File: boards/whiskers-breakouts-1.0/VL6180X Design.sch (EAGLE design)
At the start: 12 parts, among them J1 FEMALE 2x3, Q3 BSS138, Q4 BSS138, U1 VL6180X, U2 MIC5225_2.8V

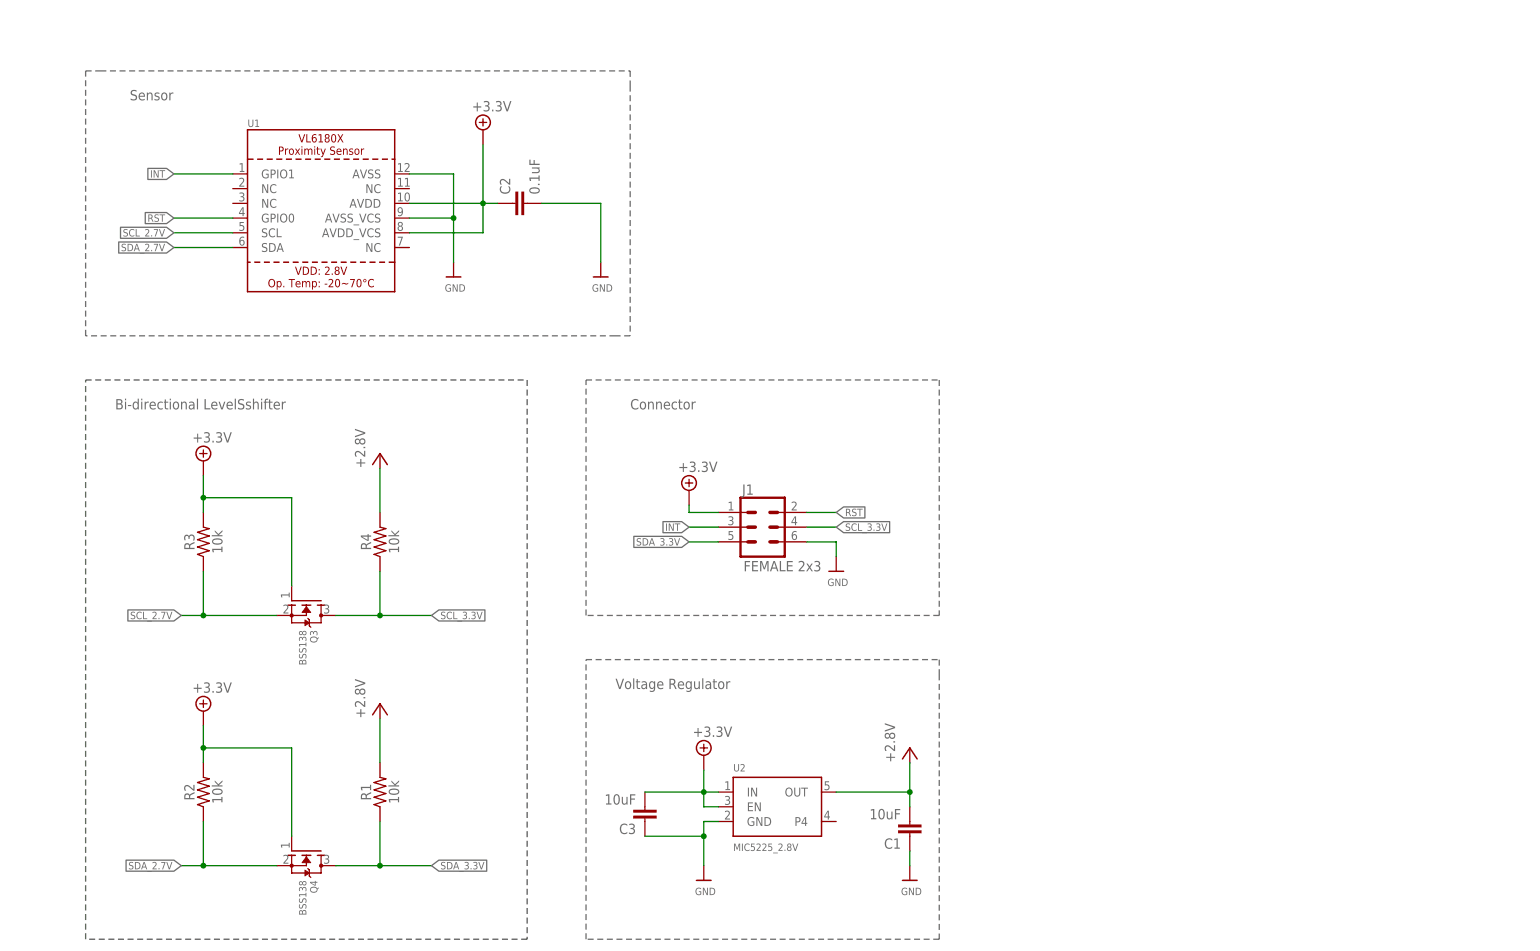
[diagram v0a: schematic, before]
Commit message: adding one more sensor
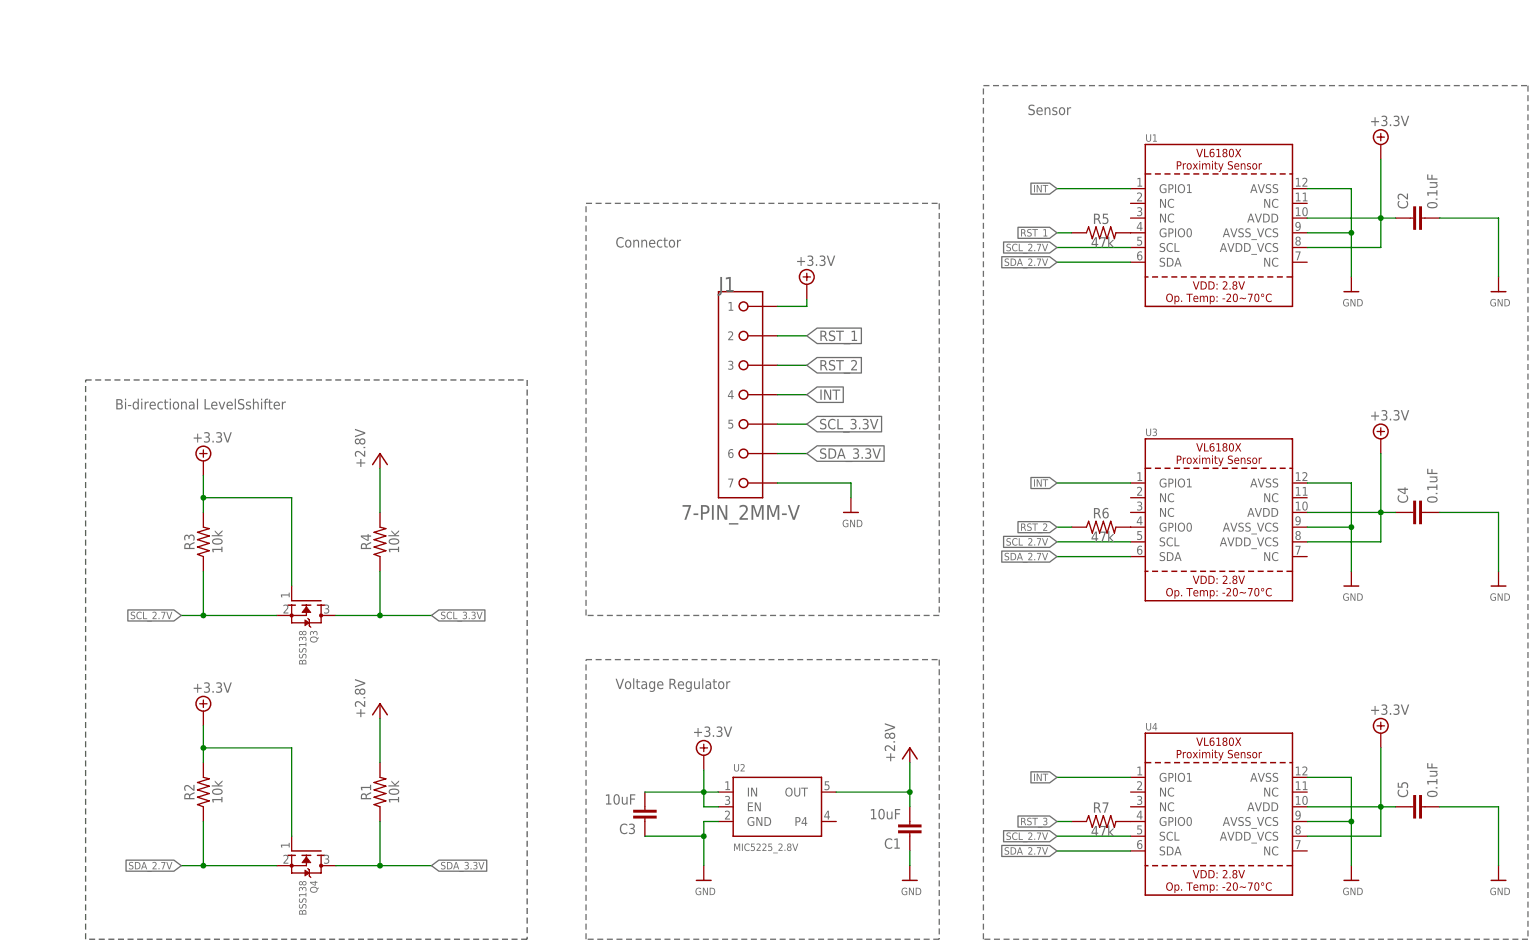
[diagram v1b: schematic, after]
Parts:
- added C4, C5: 0.1uF, SparkFun-Capacitors:1.0NF/1000PF-0603-50V-10%
- added R5, R6, R7: 47k, SparkFun-Resistors:0.05OHM-0603-1/5W-1%
- added U3, U4: VL6180X, microbuilder:VL6180X
- J1: value FEMALE 2x3 -> 7-PIN_2MM-V; device SparkFun-Connectors:CONN_03X2FEMALE -> RoboJackets-Connectors:7-PIN_2MM-V
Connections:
- removed net RST: J1.2, U1.GPIO0
- new net N$1: R5.2, U1.GPIO0
- new net N$2: R6.2, U3.GPIO0
- new net N$3: R7.2, U4.GPIO0
- new net RST_1: J1.2, R5.1
- new net RST_2: J1.3, R6.1
- new net RST_3: R7.1
- net +3.3V: now also C4.1, C5.1, U3.AVDD, U3.AVDD_VCS, U4.AVDD, U4.AVDD_VCS
- net GND: now also C4.2, C5.2, J1.7, U3.AVSS, U3.AVSS_VCS, U4.AVSS, U4.AVSS_VCS; no longer J1.6
- net INT: now also J1.4, U3.GPIO1, U4.GPIO1; no longer J1.3
- net SCL_2.7V: now also U3.SCL, U4.SCL
- net SCL_3.3V: now also J1.5; no longer J1.4
- net SDA_2.7V: now also U3.SDA, U4.SDA
- net SDA_3.3V: now also J1.6; no longer J1.5
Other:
- moved on the sheet: C2, U1

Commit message: latest
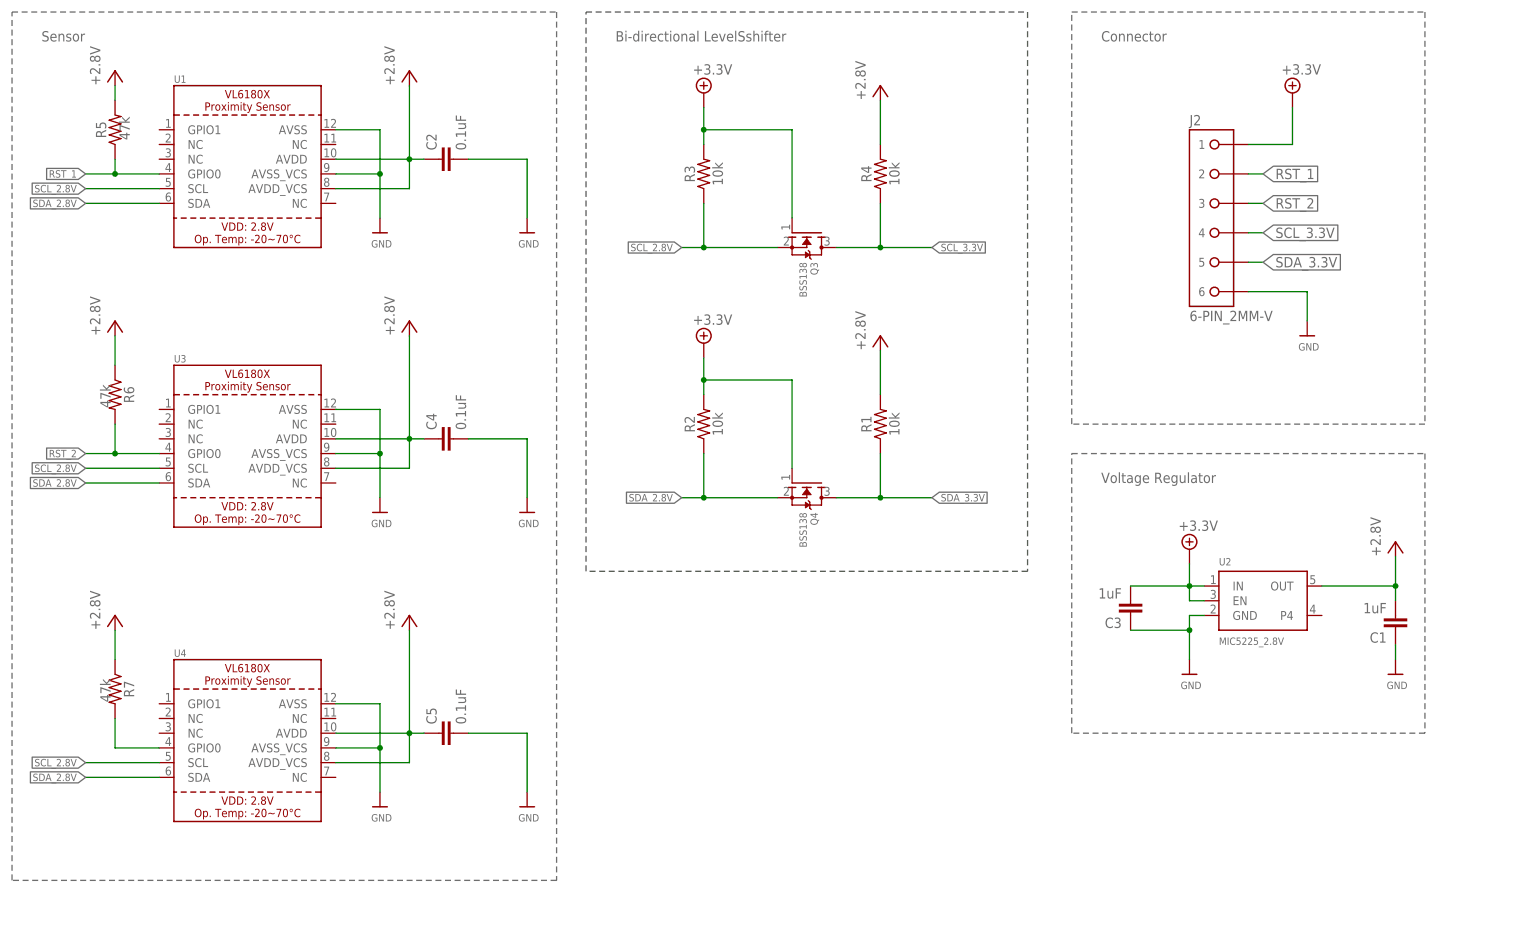
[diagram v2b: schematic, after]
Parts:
- removed J1: 7-PIN_2MM-V, RoboJackets-Connectors:7-PIN_2MM-V
- added J2: 6-PIN_2MM-V, RoboJackets-Connectors:6-PIN_2MM-V
- C1, C3: value 10uF -> 1uF
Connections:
- net SCL_2.7V renamed SCL_2.8V
- net SDA_2.7V renamed SDA_2.8V
- removed net INT: J1.4, U1.GPIO1, U3.GPIO1, U4.GPIO1
- removed net N$1: R5.2, U1.GPIO0
- removed net N$2: R6.2, U3.GPIO0
- removed net N$3: R7.2, U4.GPIO0
- net +3.3V: now also J2.1; no longer C2.1, C4.1, C5.1, J1.1, U1.AVDD, U1.AVDD_VCS, U3.AVDD, U3.AVDD_VCS, U4.AVDD, U4.AVDD_VCS
- net GND: now also J2.6; no longer J1.7
- net RST_1: now also J2.2, U1.GPIO0; no longer J1.2
- net RST_2: now also J2.3, R6.2, U3.GPIO0; no longer J1.3, R6.1
- net RST_3: now also R7.2, U4.GPIO0; no longer R7.1
- net SCL_3.3V: now also J2.4; no longer J1.5
- net SDA_3.3V: now also J2.5; no longer J1.6
- net VCC: now also C2.1, C4.1, C5.1, R5.2, R6.1, R7.1, U1.AVDD, U1.AVDD_VCS, U3.AVDD, U3.AVDD_VCS, U4.AVDD, U4.AVDD_VCS
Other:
- moved on the sheet: C1, C2, C3, C4, C5, Q3, Q4, R1, R2, R3, R4, R5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
